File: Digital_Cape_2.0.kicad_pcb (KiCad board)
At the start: 2 copper layers, 57.2 x 63.5 mm, 15 parts, among them J1 RJ45, J2 RJ45, P8 BeagleBone_Black_Header, P9 BeagleBone_Black_Header

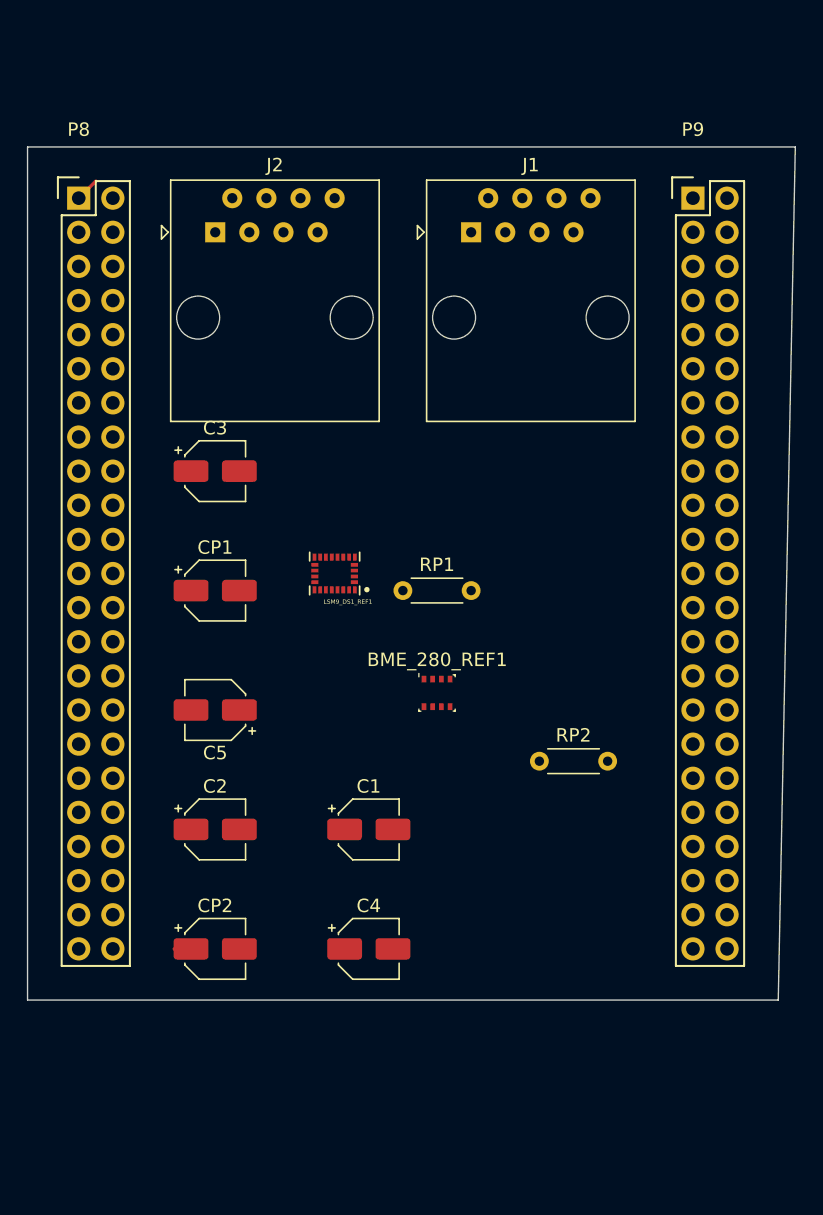
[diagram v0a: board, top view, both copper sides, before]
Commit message: Update of KiCad files
My apologies I'm still learning! Files from 02-13-2021 Hangar session
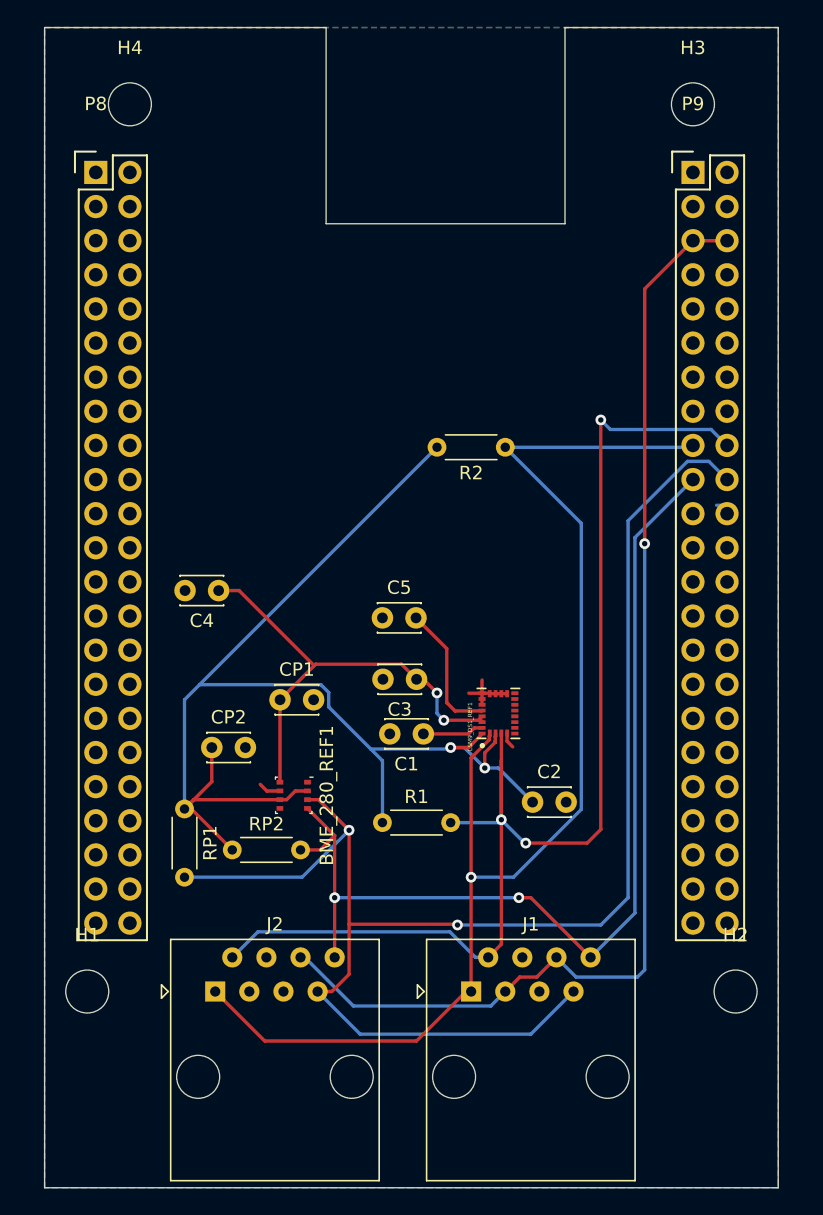
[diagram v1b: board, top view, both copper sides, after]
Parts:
- added H1: MountingHole, MountingHole:MountingHole_3.2mm_M3, F.Cu at (88.3, 121.3)
- added H2: MountingHole, MountingHole:MountingHole_3.2mm_M3, F.Cu at (136.5, 121.3)
- added H3: MountingHole, MountingHole:MountingHole_3.2mm_M3, F.Cu at (133.3, 55.2)
- added H4: MountingHole, MountingHole:MountingHole_3.2mm_M3, F.Cu at (91.4, 55.2)
- added R1: 4.7k, Resistor_THT:R_Axial_DIN0204_L3.6mm_D1.6mm_P5.08mm_Horizontal, F.Cu at (110.2, 108.7)
- added R2: 4.7k, Resistor_THT:R_Axial_DIN0204_L3.6mm_D1.6mm_P5.08mm_Horizontal, F.Cu at (119.4, 80.8)
- C1, C2, C3, C4, C5, CP1, CP2: footprint Capacitor_SMD:CP_Elec_4x4.5 -> Capacitor_THT:C_Disc_D3.0mm_W2.0mm_P2.50mm
- moved J1 56.5 mm to (116.8, 121.3)
- moved J2 56.5 mm to (97.8, 121.3)
- moved C4 28.9 mm to (98.0, 91.4), turned to 180 degrees
- moved RP2 23.8 mm to (99.1, 110.7)
- moved C2 23.7 mm to (121.4, 107.2)
- moved RP1 23.0 mm to (95.5, 107.7), turned to 270 degrees
- moved C3 21.6 mm to (112.8, 98.0), turned to 180 degrees
- moved LSM9_DS1_REF1 16.0 mm to (118.9, 100.6), turned to 90 degrees
- moved CP2 15.0 mm to (97.5, 103.1)
- moved C5 14.2 mm to (110.2, 93.5), turned to 0 degrees
- moved BME_280_REF1 13.1 mm to (103.6, 106.7), turned to 270 degrees
- moved CP1 9.45 mm to (102.6, 99.6)
- moved C1 8.19 mm to (113.3, 102.1), turned to 180 degrees
- moved P8 2.30 mm to (88.9, 60.3)
- moved P9 1.91 mm to (133.3, 60.3)
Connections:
- BME_280_REF1 pad 5: Net-(BME_280_REF1-Pad5) -> GND
- J1 pad 4: /GND1 -> GND
- J1 pad 5: /GND2 -> GND
- J2 pad 4: /GND1 -> GND
- J2 pad 5: /GND2 -> GND
- LSM9_DS1_REF1 pad 5: Net-(LSM9_DS1_REF1-Pad5) -> GND
- P8 pad 1: GNDD -> GND
- P8 pad 2: GNDD -> GND
- P9 pad 1: GNDD -> GND
- P9 pad 2: GNDD -> GND
- P9 pad 34: GNDA_ADC -> GND
- P9 pad 43: GNDD -> GND
- P9 pad 44: GNDD -> GND
- P9 pad 45: GNDD -> GND
- P9 pad 46: GNDD -> GND
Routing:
- net /I2C2_SDA: track 0.78 -> 112.5 mm, vias 0 -> 2
- net /I2C1_SCL: track 0.00 -> 95.5 mm, vias 0 -> 1
- net /I2C1_SDA: track 0.00 -> 95.2 mm, vias 0 -> 3
- net /Vdd_IO: track 0.72 -> 95.4 mm, vias 0 -> 2
- net +5V: track 0.00 -> 87.7 mm, vias 0 -> 1
- net /I2C2_SCL: track 0.00 -> 74.6 mm, vias 0 -> 2
- net /Vdd: track 0.00 -> 34.7 mm, vias 0 -> 2
- net Net-(C5-Pad2): track 0.00 -> 10.2 mm
- net GND: track 0.00 -> 7.73 mm
- net Net-(C1-Pad1): track 0.00 -> 4.55 mm
- net GNDD: track 2.52 -> 0.00 mm
- net /uart2_rxd: track 0.00 -> 0.78 mm
- added copper zone on B.Cu, net GND
- added copper zone on F.Cu, net GND
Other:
- board size 57.2 x 63.5 mm -> 54.6 x 86.4 mm
- net class Default: clearance 0.2 -> 0.127
- rule trace_clearance: 0.2 -> 0.127
